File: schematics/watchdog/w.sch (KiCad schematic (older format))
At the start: 19 parts, among them J1 VOUT 3V, J2 Power IN, J3 I2C, J4 VOUT 5V, J5 Conn_01x08_MountingPin, Q1 IRF4905, Q2 2N2219, Q3 IRF4905, Q4 2N2219, U1 ATtiny85-20PU, U2 AMS1117

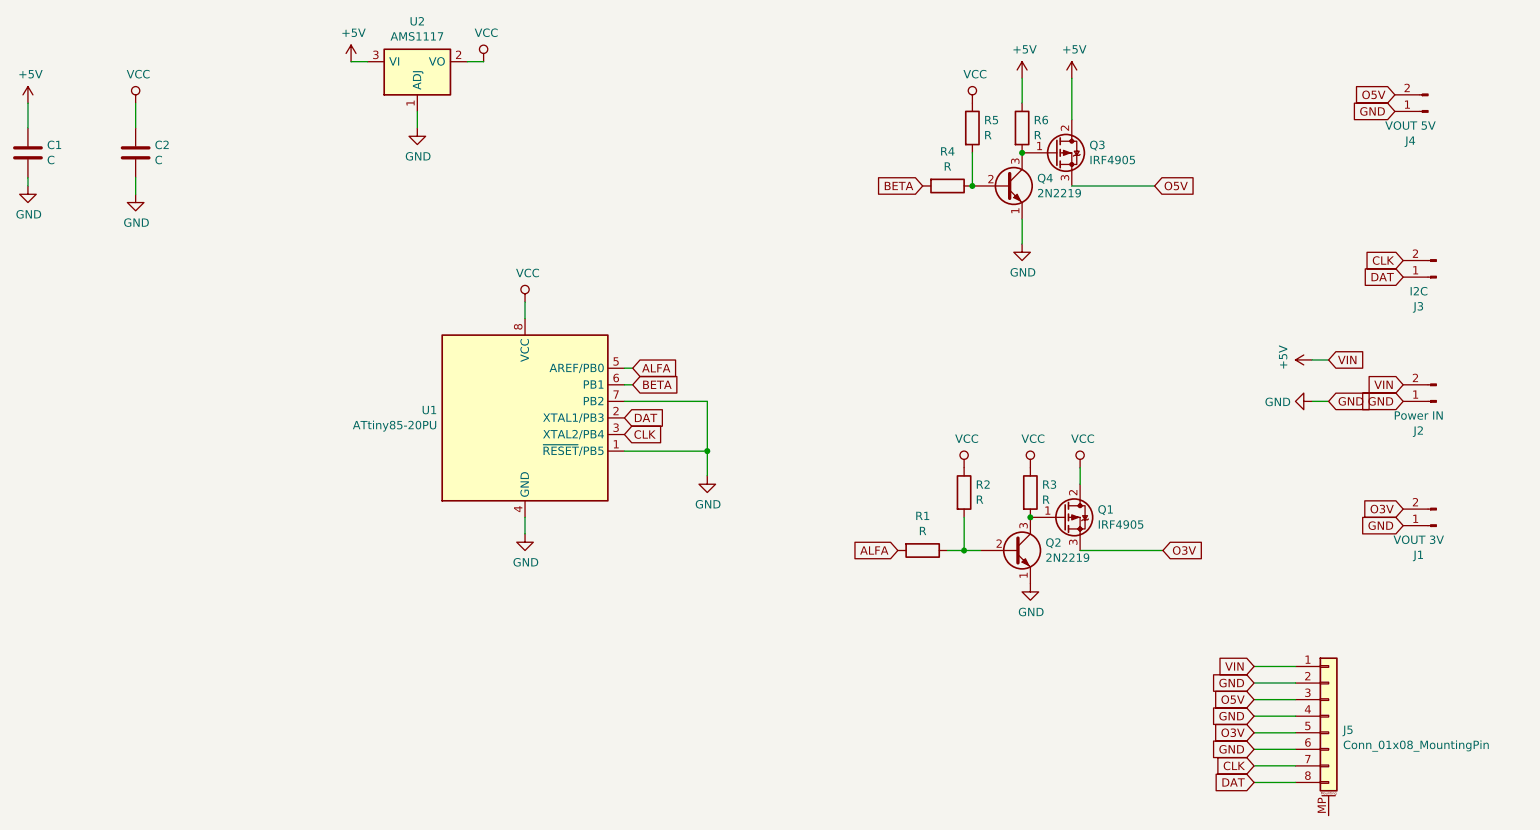
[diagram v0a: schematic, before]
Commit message: Aktualizacja schematu.
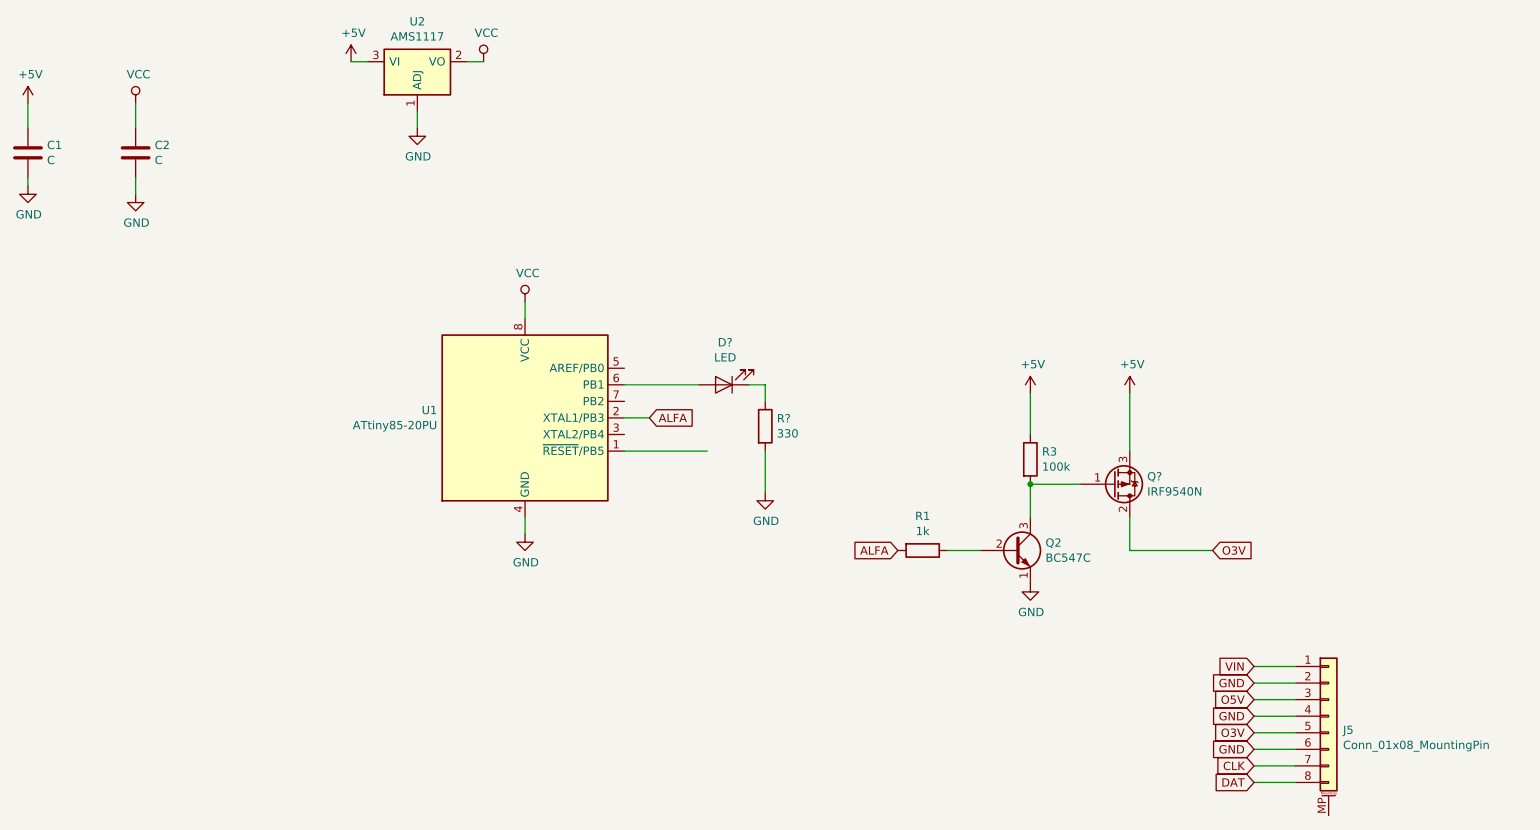
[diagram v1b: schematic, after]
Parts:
- removed J1: VOUT 3V, Connector_PinHeader_2.54mm:PinHeader_1x01_P2.54mm_Horizontal, symbol Connector:Conn_01x02_Male
- removed J2: Power IN, Connector_PinHeader_2.54mm:PinHeader_1x01_P2.54mm_Horizontal, symbol Connector:Conn_01x02_Male
- removed J3: I2C, Connector_PinHeader_2.54mm:PinHeader_1x01_P2.54mm_Horizontal, symbol Connector:Conn_01x02_Male
- removed J4: VOUT 5V, Connector_PinHeader_2.54mm:PinHeader_1x01_P2.54mm_Horizontal, symbol Connector:Conn_01x02_Male
- removed Q1, Q3: IRF4905, Package_TO_SOT_THT:TO-220-3_Vertical, symbol Transistor_FET:IRF4905
- removed Q4: 2N2219, Package_TO_SOT_THT:TO-39-3, symbol Transistor_BJT:2N2219
- removed R2, R4, R5, R6: R, Resistor_THT:R_Axial_DIN0204_L3.6mm_D1.6mm_P1.90mm_Vertical, symbol Device:R
- added D?: LED, symbol Device:LED
- added Q?: IRF9540N, Package_TO_SOT_THT:TO-220-3_Vertical, symbol Transistor_FET:IRF9540N
- added R?: 330, symbol Device:R
- Q2: value 2N2219 -> BC547C
- R1: value R -> 1k
- R3: value R -> 100k
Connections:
- net +5V: now also R3.1, Q?.3 (S); no longer J5.1 (Pin_1)
- net ALFA: now also U1.2 (XTAL1/PB3); no longer U1.5 (AREF/PB0)
- net CLK: no longer U1.3 (XTAL2/PB4)
- net DAT: no longer U1.2 (XTAL1/PB3)
- net GND: now also R?.2; no longer U1.1 (~RESET~/PB5), U1.7 (PB2)
- net O3V: now also Q?.2 (D)
- net VCC: no longer R3.1
- net at Q2.3 (C), R3.2: now also Q?.1 (G)
- net BETA: no longer names the net of U1.6 (PB1)
- net BETA: now also D?.2 (A)
- new net: D?.1 (K), R?.1
- new net VIN: J5.1 (Pin_1)
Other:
- moved on the sheet: R3
